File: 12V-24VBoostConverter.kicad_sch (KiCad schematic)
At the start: 19 parts, among them IC1 TPS613771RYHR

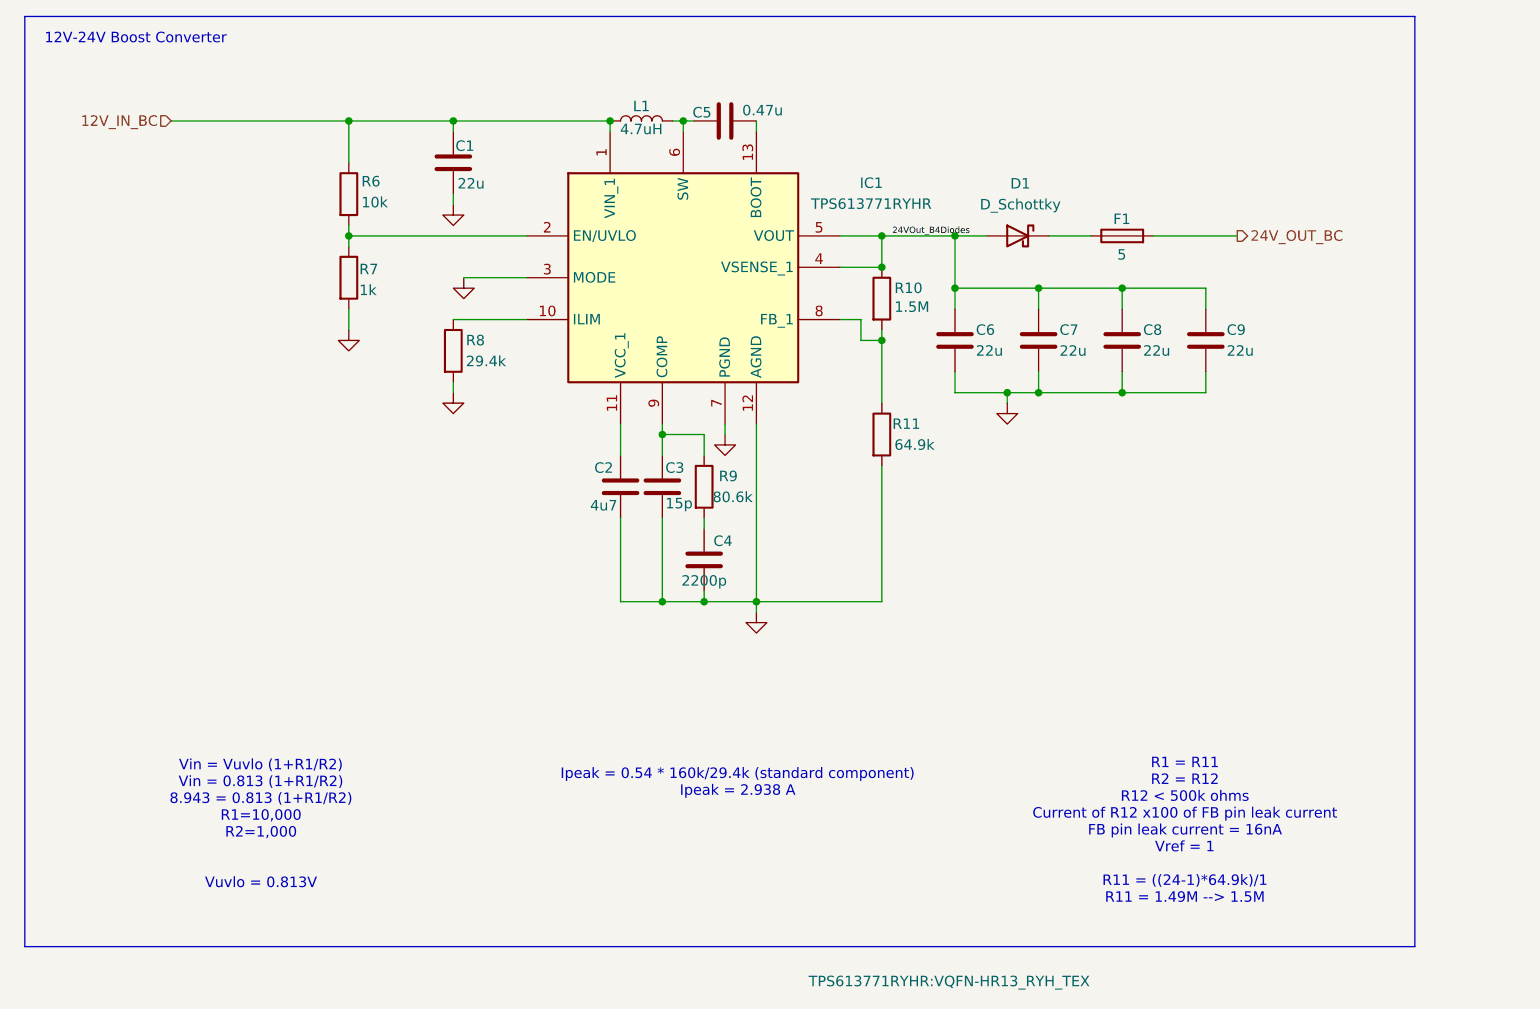
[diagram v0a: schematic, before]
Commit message: RevA11 for review
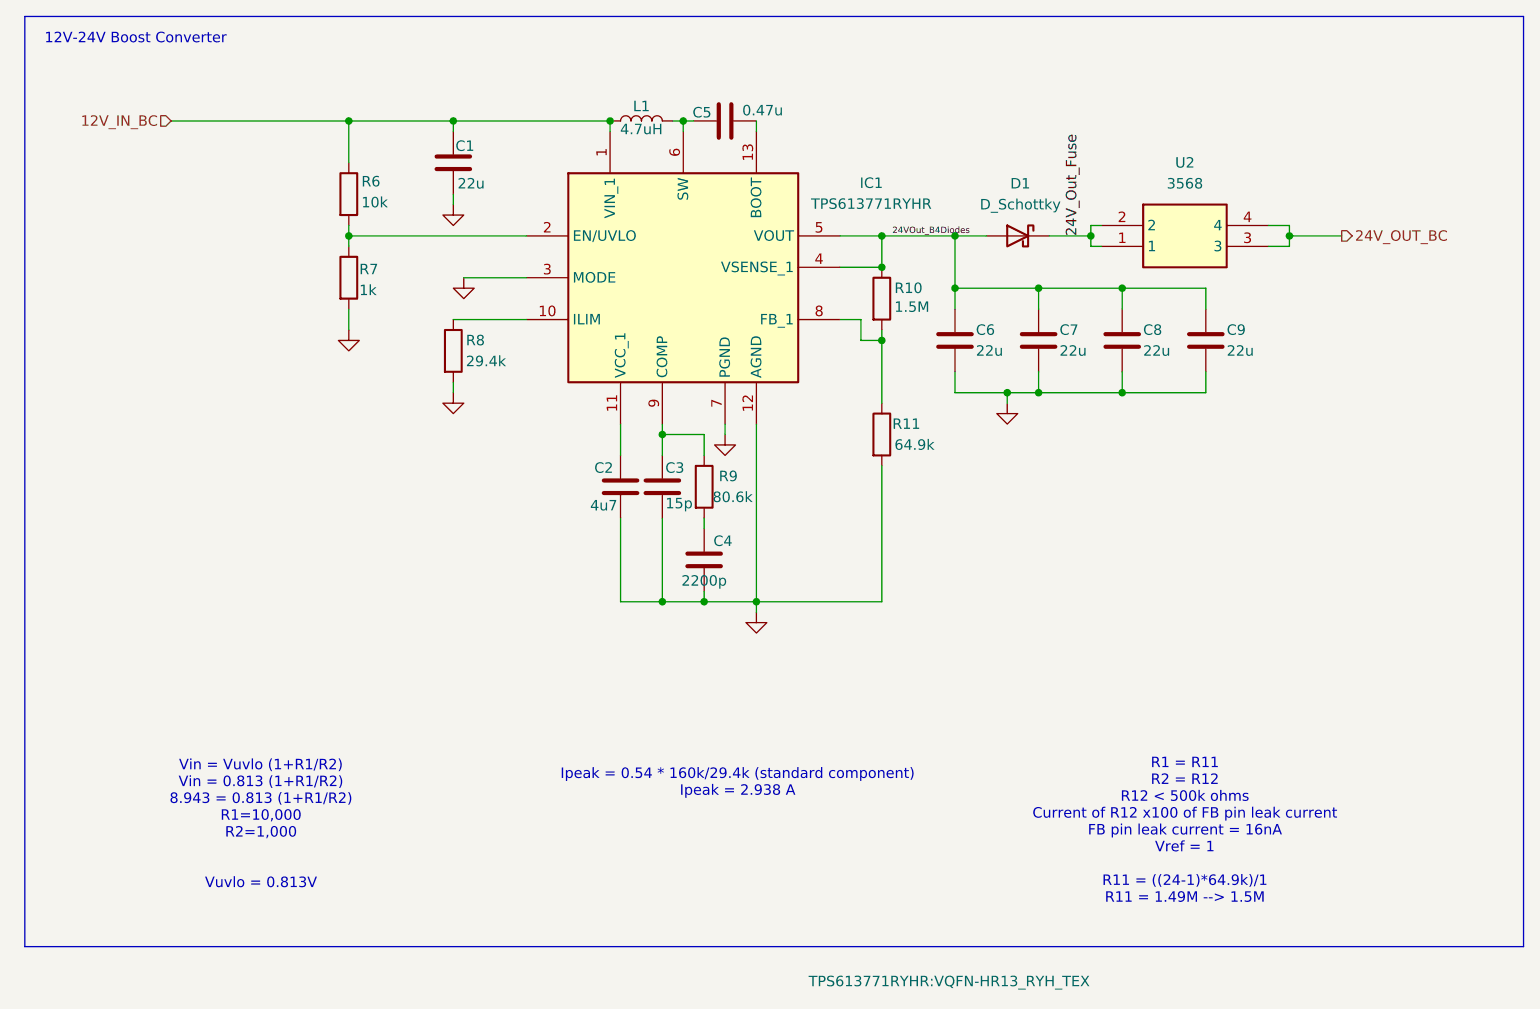
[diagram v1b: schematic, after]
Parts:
- removed F1: 5, Fuse:Fuse_0805_2012Metric, symbol Device:Fuse
- added U2: 3568, 3568:3568, symbol 3568:3568
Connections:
- net 24V_OUT_BC: now also U2.3, U2.4
- net 24V_Out_Fuse: now reaches D1.1 (K)
- net 24V_Out_Fuse: now also U2.1, U2.2
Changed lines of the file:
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@@
 	(rectangle
 		(start 15.24 16.51)
-		(end 184.15 129.54)
+		(end 197.358 129.54)
 		(stroke
 			(width 0)
@@
 	)
 	(junction
+		(at 144.78 43.18)
+		(diameter 0)
+		(color 0 0 0 0)
+	)
+	(junction
 		(at 92.71 67.31)
 		(diameter 0)
@@
 	)
 	(junction
+		(at 168.91 43.18)
+		(diameter 0)
+		(color 0 0 0 0)
+	)
+	(junction
 		(at 104.14 87.63)
 		(diameter 0)
@@
 	(wire
 		(pts
-			(xy 152.4 43.18) (xy 162.56 43.18)
+			(xy 168.91 43.18) (xy 175.26 43.18)
 		)
 		(stroke
@@
 	(wire
 		(pts
+			(xy 144.78 43.18) (xy 144.78 41.91)
+		)
+		(stroke
+			(width 0)
+			(type default)
+		)
+	)
+	(wire
+		(pts
 			(xy 104.14 66.04) (xy 104.14 87.63)
 		)
@@
 	(wire
 		(pts
+			(xy 144.78 44.45) (xy 144.78 43.18)
+		)
+		(stroke
+			(width 0)
+			(type default)
+		)
+	)
+	(wire
+		(pts
 			(xy 119.38 71.12) (xy 119.38 87.63)
 		)
@@
 	(wire
 		(pts
+			(xy 146.05 44.45) (xy 144.78 44.45)
+		)
+		(stroke
+			(width 0)
+			(type default)
+		)
+	)
+	(wire
+		(pts
 			(xy 67.31 29.21) (xy 67.31 30.48)
 		)
@@
 	(wire
 		(pts
+			(xy 166.37 44.45) (xy 168.91 44.45)
+		)
+		(stroke
+			(width 0)
+			(type default)
+		)
+	)
+	(wire
+		(pts
 			(xy 97.79 67.31) (xy 97.79 69.85)
 		)
@@
 	(wire
 		(pts
+			(xy 168.91 41.91) (xy 168.91 43.18)
+		)
+		(stroke
+			(width 0)
+			(type default)
+		)
+	)
+	(wire
+		(pts
 			(xy 119.38 43.18) (xy 128.27 43.18)
 		)
@@
 	(wire
 		(pts
+			(xy 166.37 41.91) (xy 168.91 41.91)
+		)
+		(stroke
+			(width 0)
+			(type default)
+		)
+	)
+	(wire
+		(pts
 			(xy 95.25 29.21) (xy 95.25 30.48)
 		)
@@
 	(wire
 		(pts
+			(xy 168.91 44.45) (xy 168.91 43.18)
+		)
+		(stroke
+			(width 0)
+			(type default)
+		)
+	)
+	(wire
+		(pts
 			(xy 92.71 87.63) (xy 97.79 87.63)
 		)
@@
 	(wire
 		(pts
+			(xy 144.78 41.91) (xy 146.05 41.91)
+		)
+		(stroke
+			(width 0)
+			(type default)
+		)
+	)
+	(wire
+		(pts
 			(xy 87.63 66.04) (xy 87.63 69.85)
 		)
@@
 		)
 	)
+	(label "24V_Out_Fuse"
+		(at 143.51 43.18 90)
+		(effects
+			(font
+				(size 1.27 1.27)
+			)
+			(justify left bottom)
+		)
+	)
 	(label "24VOut_B4Diodes"
 		(at 120.65 43.18 0)
@@
 	(hierarchical_label "24V_OUT_BC"
 		(shape output)
-		(at 162.56 43.18 0)
+		(at 175.26 43.18 0)
 		(effects
 			(font
@@
 	)
 	(symbol
-		(lib_id "Device:Fuse")
-		(at 148.59 43.18 90)
-		(unit 1)
-		(exclude_from_sim no)
-		(in_bom yes)
-		(on_board yes)
-		(dnp no)
-		(property "Reference" "F1"
-			(at 149.606 41.148 90)
-			(effects
-				(font
-					(size 1.27 1.27)
-				)
-				(justify left)
-			)
-		)
-		(property "Value" "5"
-			(at 149.098 45.466 90)
-			(effects
-				(font
-					(size 1.27 1.27)
-				)
-				(justify left)
-			)
-		)
-		(property "Footprint" "Fuse:Fuse_0805_2012Metric"
-			(at 148.59 44.958 90)
-			(effects
-				(font
-					(size 1.27 1.27)
-				)
-				(hide yes)
-			)
-		)
-		(property "Datasheet" "~"
-			(at 148.59 43.18 0)
-			(effects
-				(font
-					(size 1.27 1.27)
-				)
-				(hide yes)
-			)
-		)
-		(property "Description" "Fuse"
-			(at 148.59 43.18 0)
-			(effects
-				(font
-					(size 1.27 1.27)
-				)
-				(hide yes)
-			)
-		)
-		(property "MANUFACTURER" ""
-			(at 148.59 43.18 90)
-			(effects
-				(font
-					(size 1.27 1.27)
-				)
-				(hide yes)
-			)
-		)
-		(property "PARTREV" ""
-			(at 148.59 43.18 90)
-			(effects
-				(font
-					(size 1.27 1.27)
-				)
-				(hide yes)
-			)
-		)
-		(property "STANDARD" ""
-			(at 148.59 43.18 90)
-			(effects
-				(font
-					(size 1.27 1.27)
-				)
-				(hide yes)
-			)
-		)
-		(pin "1"
-		)
-		(pin "2"
-		)
-		(instances
-			(project "PS-ChargerInterfacePCB"
-				(path "/d45494af-ff47-4110-bed2-dd613b557244/a5946dd4-2cac-491d-9b85-f213ab9011e7"
-					(reference "F1")
-					(unit 1)
-				)
-			)
-		)
-	)
-	(symbol
 		(lib_id "power:GND")
 		(at 104.14 88.9 0)
@@
 					(unit 1)
 				)
+			)
+		)
+	)
+	(symbol
+		(lib_id "3568:3568")
+		(at 146.05 41.91 0)
+		(unit 1)
+		(exclude_from_sim no)
+		(in_bom yes)
+		(on_board yes)
+		(dnp no)
+		(fields_autoplaced yes)
+		(property "Reference" "U2"
+			(at 156.21 34.29 0)
+			(effects
+				(font
+					(size 1.27 1.27)
+				)
+			)
+		)
+		(property "Value" "3568"
+			(at 156.21 36.83 0)
+			(effects
+				(font
+					(size 1.27 1.27)
+				)
+			)
+		)
+		(property "Footprint" "3568:3568"
+			(at 162.56 136.83 0)
+			(effects
+				(font
+					(size 1.27 1.27)
+				)
+				(justify left top)
+				(hide yes)
+			)
+		)
+		(property "Datasheet" "https://www.keyelco.com/userAssets/file/M65p42.pdf"
+			(at 162.56 236.83 0)
+			(effects
+				(font
+					(size 1.27 1.27)
+				)
+				(justify left top)
+				(hide yes)
+			)
+		)
+		(property "Description" "Fuse Holder 30A 500V 1 Circuit Blade Through Hole"
+			(at 146.05 41.91 0)
+			(effects
+				(font
+					(size 1.27 1.27)
+				)
+				(hide yes)
+			)
+		)
+		(property "Height" "7.5"
+			(at 162.56 436.83 0)
+			(effects
+				(font
+					(size 1.27 1.27)
+				)
+				(justify left top)
+				(hide yes)
+			)
+		)
+		(property "Mouser Part Number" "534-3568"
+			(at 162.56 536.83 0)
+			(effects
+				(font
+					(size 1.27 1.27)
+				)
+				(justify left top)
+				(hide yes)
+			)
+		)
+		(property "Mouser Price/Stock" "https://www.mouser.co.uk/ProductDetail/Keystone-Electronics/3568?qs=fP5bVVCrK%2Fd7nbA%2FPpwnKw%3D%3D"
+			(at 162.56 636.83 0)
+			(effects
+				(font
+					(size 1.27 1.27)
+				)
+				(justify left top)
+				(hide yes)
+			)
+		)
+		(property "Manufacturer_Name" "Keystone Electronics"
+			(at 162.56 736.83 0)
+			(effects
+				(font
+					(size 1.27 1.27)
+				)
+				(justify left top)
+				(hide yes)
+			)
+		)
+		(property "Manufacturer_Part_Number" "3568"
+			(at 162.56 836.83 0)
+			(effects
+				(font
+					(size 1.27 1.27)
+				)
+				(justify left top)
+				(hide yes)
+			)
+		)
+		(property "Distrbutor Link" "https://www.digikey.com/en/products/detail/keystone-electronics/3568/2137306"
+			(at 146.05 41.91 0)
+			(effects
+				(font
+					(size 1.27 1.27)
+				)
+				(hide yes)
+			)
+		)
+		(property "Manufacturer" "Keystone Electronics"
+			(at 146.05 41.91 0)
+			(effects
+				(font
+					(size 1.27 1.27)
+				)
+				(hide yes)
+			)
+		)
+		(pin "3"
+		)
+		(pin "4"
+		)
+		(pin "1"
+		)
+		(pin "2"
+		)
+		(instances
+			(project ""
+				(path "/d45494af-ff47-4110-bed2-dd613b557244/a5946dd4-2cac-491d-9b85-f213ab9011e7"
+					(reference "U2")
+					(unit 1)
+				)

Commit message: Added BOM, CPL
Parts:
- C1, C6, C7, C8, C9: Manufacturer_Part_Number GRM21BR61E226ME44L -> (none); P/N (none) -> GRM21BR61E226ME44L
- C2: Manufacturer_Part_Number 08055D475KAT4A -> (none); P/N (none) -> 08055D475KAT4A
- C3: Manufacturer_Part_Number 0603N150J250CT -> (none); P/N (none) -> 0603N150J250CT
- C4: Manufacturer_Part_Number GCJ188R71E222KA01D -> (none); P/N (none) -> GCJ188R71E222KA01D
- C5: Manufacturer_Part_Number 0603B474K500CT -> (none); P/N (none) -> 0603B474K500CT
- D1: Manufacturer_Part_Number SK32A-LTP -> (none); P/N (none) -> SK32A-LTP
- IC1: Manufacturer_Part_Number TPS613771RYHR -> (none); P/N (none) -> TPS613771RYHR
- L1: Distrbutor Link https://www.digikey.com/en/products/detail/coilcraft/XGL402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 -> https://www.digikey.com/en/products/detail/coilcraft/xgl402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; Manufacturer_Part_Number XGL4020-472MEC -> (none); P/N (none) -> XGL4020-472MEC
- R10: Manufacturer_Part_Number CRCW06031M50JNTA -> (none); P/N (none) -> CRCW06031M50JNTA
- R11: Manufacturer_Part_Number CRCW060364K9FKEA -> (none); P/N (none) -> CRCW060364K9FKEA
- R6: Manufacturer_Part_Number CRCW060310K0FKEI -> (none); P/N (none) -> CRCW060310K0FKEI
- R7: Manufacturer_Part_Number CRCW06031K00FKEI -> (none); P/N (none) -> CRCW06031K00FKEI
- R8: Manufacturer_Part_Number CRCW060329K4FKEAC -> (none); P/N (none) -> CRCW060329K4FKEAC
- R9: Manufacturer_Part_Number CRCW060380K6FKEA -> (none); P/N (none) -> CRCW060380K6FKEA
- U2: Distrbutor Link https://www.digikey.com/en/products/detail/keystone-electro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 -> https://www.mouser.com/ProductDetail/Keystone-Electronics/3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; Manufacturer_Part_Number 3568 -> (none); P/N (none) -> 3568
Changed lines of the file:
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@@
 			)
 		)
-		(property "Manufacturer_Part_Number" "GCJ188R71E222KA01D"
+		(property "P/N" "GCJ188R71E222KA01D"
 			(at 97.79 82.55 0)
 			(effects
@@
 			)
 		)
-		(property "Manufacturer_Part_Number" "08055D475KAT4A"
+		(property "P/N" "08055D475KAT4A"
 			(at 87.63 73.66 0)
 			(effects
@@
 			)
 		)
-		(property "Manufacturer_Part_Number" "0603N150J250CT"
+		(property "P/N" "0603N150J250CT"
 			(at 92.71 73.66 0)
 			(effects
@@
 			)
 		)
-		(property "Manufacturer_Part_Number" "CRCW06031K00FKEI"
+		(property "P/N" "CRCW06031K00FKEI"
 			(at 54.61 48.26 0)
 			(effects
@@
 			)
 		)
-		(property "Manufacturer_Part_Number" "CRCW060310K0FKEI"
+		(property "P/N" "CRCW060310K0FKEI"
 			(at 54.61 38.1 0)
 			(effects
@@
 			)
 		)
-		(property "Manufacturer_Part_Number" "CRCW06031M50JNTA"
+		(property "P/N" "CRCW06031M50JNTA"
 			(at 119.38 50.8 0)
 			(effects
@@
 			)
 		)
-		(property "Distrbutor Link" "https://www.digikey.com/en/products/detail/coilcraft/XGL4020-472MEC/12714544"
+		(property "Distrbutor Link" "https://www.digikey.com/en/products/detail/coilcraft/xgl4020-472mec/12714544"
 			(at 90.17 29.21 90)
 			(effects
@@
 			)
 		)
-		(property "Manufacturer_Part_Number" "XGL4020-472MEC"
+		(property "P/N" "XGL4020-472MEC"
 			(at 90.17 29.21 90)
 			(effects
@@
 			)
 		)
-		(property "Manufacturer_Part_Number" "GRM21BR61E226ME44L "
+		(property "P/N" "GRM21BR61E226ME44L "
 			(at 67.31 34.29 0)
 			(effects
@@
 			)
 		)
-		(property "Manufacturer_Part_Number" "TPS613771RYHR"
-			(at 110.49 833.02 0)
-			(effects
-				(font
-					(size 1.27 1.27)
-				)
-				(justify left top)
-				(hide yes)
-			)
-		)
 		(property "MANUFACTURER" ""
 			(at 76.2 38.1 0)
@@
 		)
 		(property "Manufacturer" "Texas Instruments"
+			(at 76.2 38.1 0)
+			(effects
+				(font
+					(size 1.27 1.27)
+				)
+				(hide yes)
+			)
+		)
+		(property "P/N" "TPS613771RYHR"
 			(at 76.2 38.1 0)
 			(effects
@@
 			)
 		)
-		(property "Manufacturer_Part_Number" "CRCW060364K9FKEA"
+		(property "P/N" "CRCW060364K9FKEA"
 			(at 119.38 67.31 0)
 			(effects
@@
 			)
 		)
-		(property "Manufacturer_Part_Number" "0603B474K500CT"
+		(property "P/N" "0603B474K500CT"
 			(at 100.33 29.21 90)
 			(effects
@@
 			)
 		)
-		(property "Manufacturer_Part_Number" "CRCW060380K6FKEA"
+		(property "P/N" "CRCW060380K6FKEA"
 			(at 97.79 73.66 0)
 			(effects
@@
 			)
 		)
-		(property "Manufacturer_Part_Number" "CRCW060329K4FKEAC"
+		(property "P/N" "CRCW060329K4FKEAC"
 			(at 67.31 57.15 0)
 			(effects
@@
 			)
 		)
-		(property "Manufacturer_Part_Number" "SK32A-LTP"
+		(property "P/N" "SK32A-LTP"
 			(at 135.89 43.18 0)
 			(effects
@@
 			)
 		)
-		(property "Manufacturer_Part_Number" "GRM21BR61E226ME44L "
+		(property "P/N" "GRM21BR61E226ME44L "
 			(at 138.43 55.88 0)
 			(effects
@@
 			)
 		)
-		(property "Manufacturer_Part_Number" "GRM21BR61E226ME44L "
+		(property "P/N" "GRM21BR61E226ME44L "
 			(at 128.27 55.88 0)
 			(effects
@@
 			)
 		)
-		(property "Manufacturer_Part_Number" "GRM21BR61E226ME44L "
+		(property "P/N" "GRM21BR61E226ME44L "
 			(at 148.59 55.88 0)
 			(effects
@@
 			)
 		)
-		(property "Manufacturer_Part_Number" "3568"
-			(at 162.56 836.83 0)
-			(effects
-				(font
-					(size 1.27 1.27)
-				)
-				(justify left top)
-				(hide yes)
-			)
-		)
-		(property "Distrbutor Link" "https://www.digikey.com/en/products/detail/keystone-electronics/3568/2137306"
+		(property "Distrbutor Link" "https://www.mouser.com/ProductDetail/Keystone-Electronics/3568?qs=fP5bVVCrK%2Fd7nbA%2FPpwnKw%3D%3D"
 			(at 146.05 41.91 0)
 			(effects
@@
 		)
 		(property "Manufacturer" "Keystone Electronics"
+			(at 146.05 41.91 0)
+			(effects
+				(font
+					(size 1.27 1.27)
+				)
+				(hide yes)
+			)
+		)
+		(property "P/N" "3568"
 			(at 146.05 41.91 0)
 			(effects
@@
 			)
 		)
-		(property "Manufacturer_Part_Number" "GRM21BR61E226ME44L "
+		(property "P/N" "GRM21BR61E226ME44L "
 			(at 158.75 55.88 0)
 			(effects
